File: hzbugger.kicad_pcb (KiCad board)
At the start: 2 copper layers, 53.5 x 26.7 mm, 57 parts, among them J1 SELF_SWD, J2 IDC, J6 GPIO, SW1 RESET_SW, SW2 BOOT0_SW, U1 STM32F103C8T6, U2 SRV05-4, U3 AMS1117-3.3, U4 HX AM 90D, Y1 8M

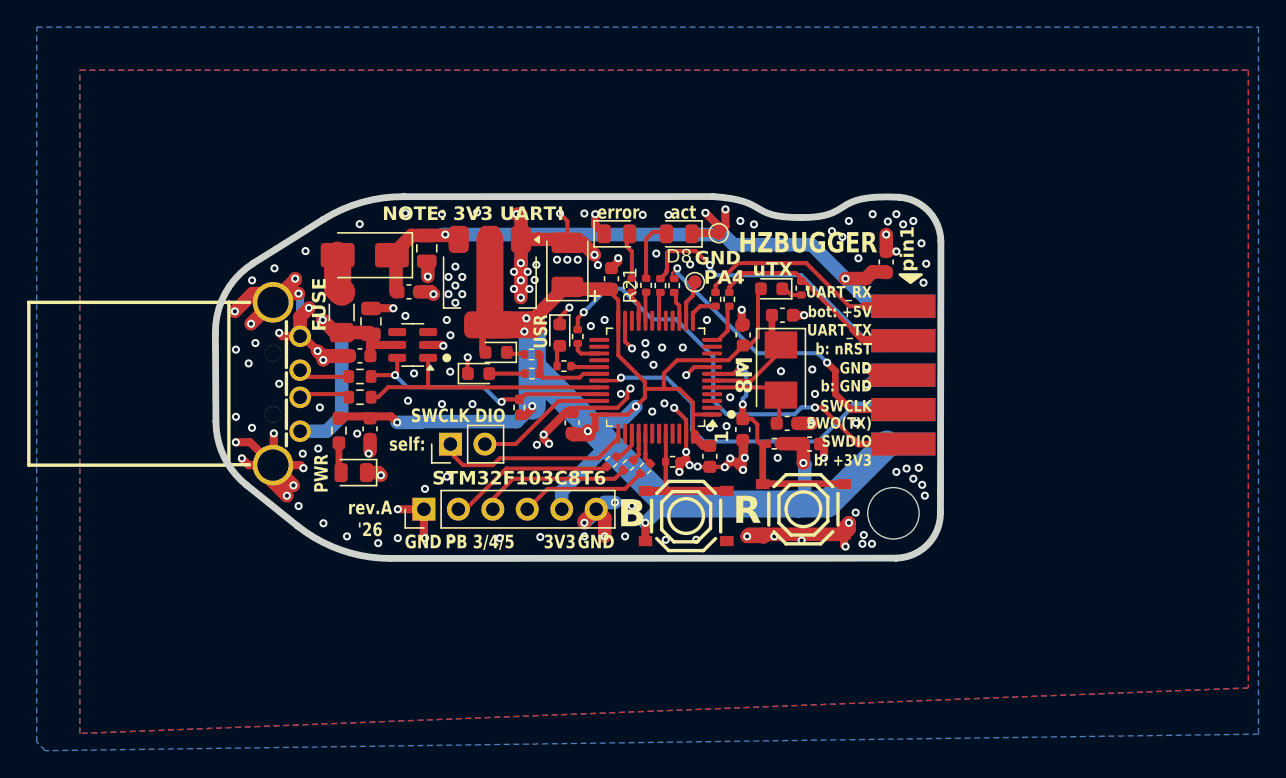
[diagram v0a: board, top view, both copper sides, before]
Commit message: form factor, mounting holes
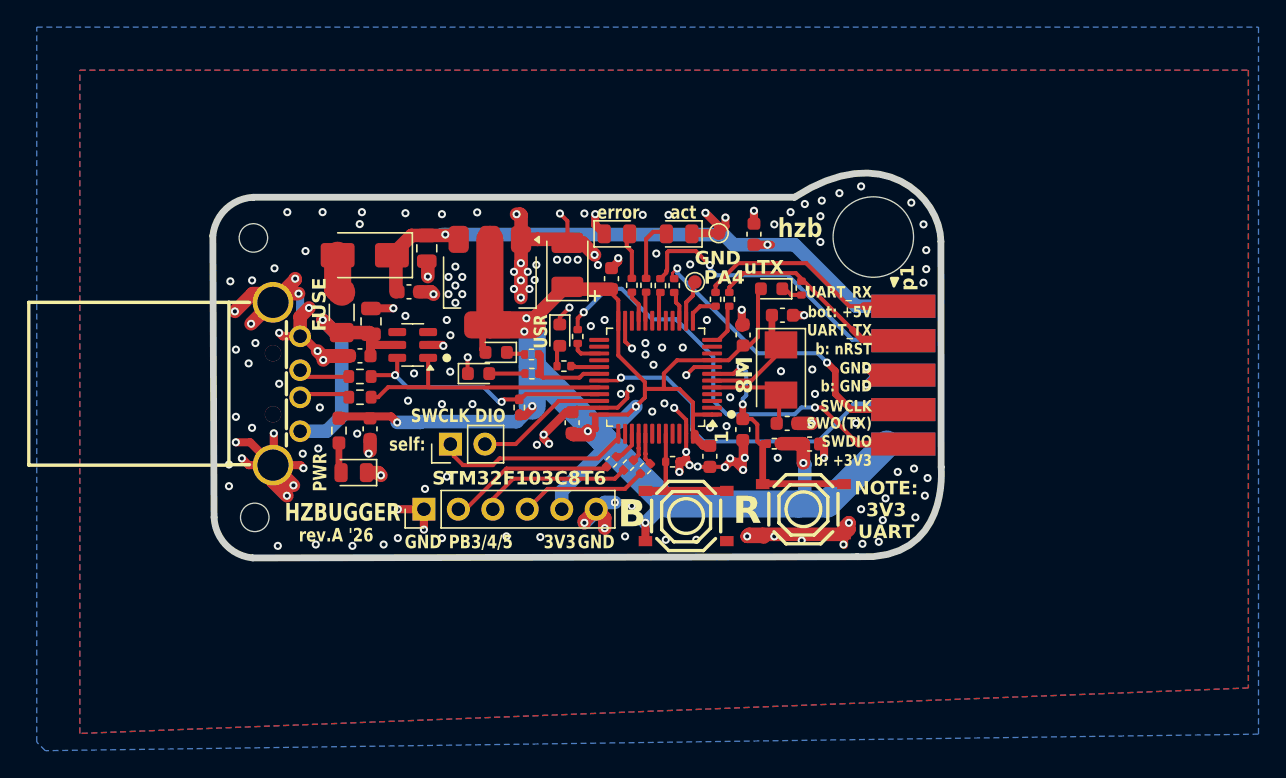
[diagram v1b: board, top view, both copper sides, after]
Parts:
- added H1: MountingHole, MountingHole:MountingHole_2.1mm, F.Cu at (103.6, 76.5)
- added H2: MountingHole_Pad, MountingHole:MountingHole_2.1mm, F.Cu at (103.7, 97.1)
- moved C14 9.96 mm to (140.5, 76.2)
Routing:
- net GND: track 144.6 -> 141.6 mm, vias 170 -> 173
- net +5V: track 48.5 -> 46.6 mm
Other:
- board size 53.5 x 26.7 mm -> 53.7 x 28.4 mm
- board text added: "NOTE: 3V3 UART"
- board text added: "PB3/4/5"
- board text added: "hzb"
- board text added: "p1"
- board text removed: "NOTE: 3V3 UART!"
- board text removed: "PB 3/4/5"
- board text removed: "pin1"
